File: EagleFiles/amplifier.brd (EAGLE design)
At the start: 100 x 80 mm, 52 parts, among them X1 736880-49

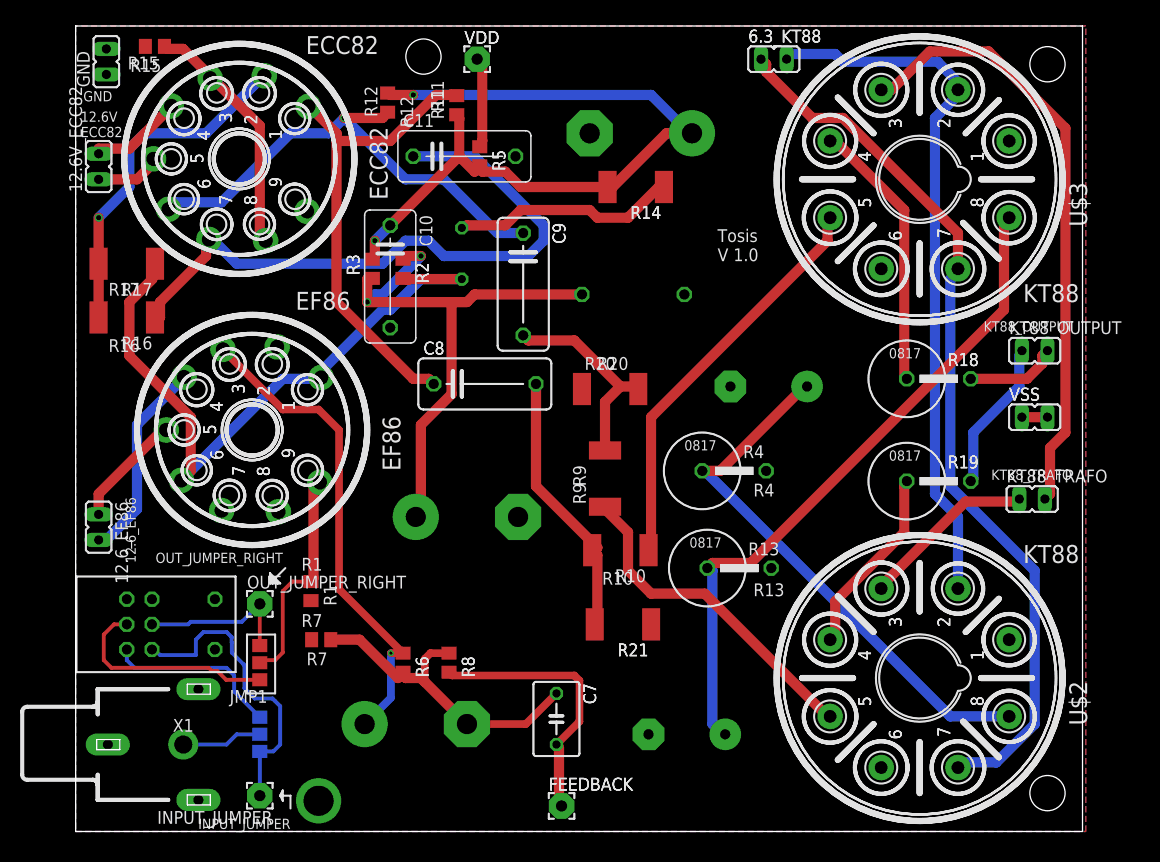
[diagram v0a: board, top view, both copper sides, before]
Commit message: last not good design.
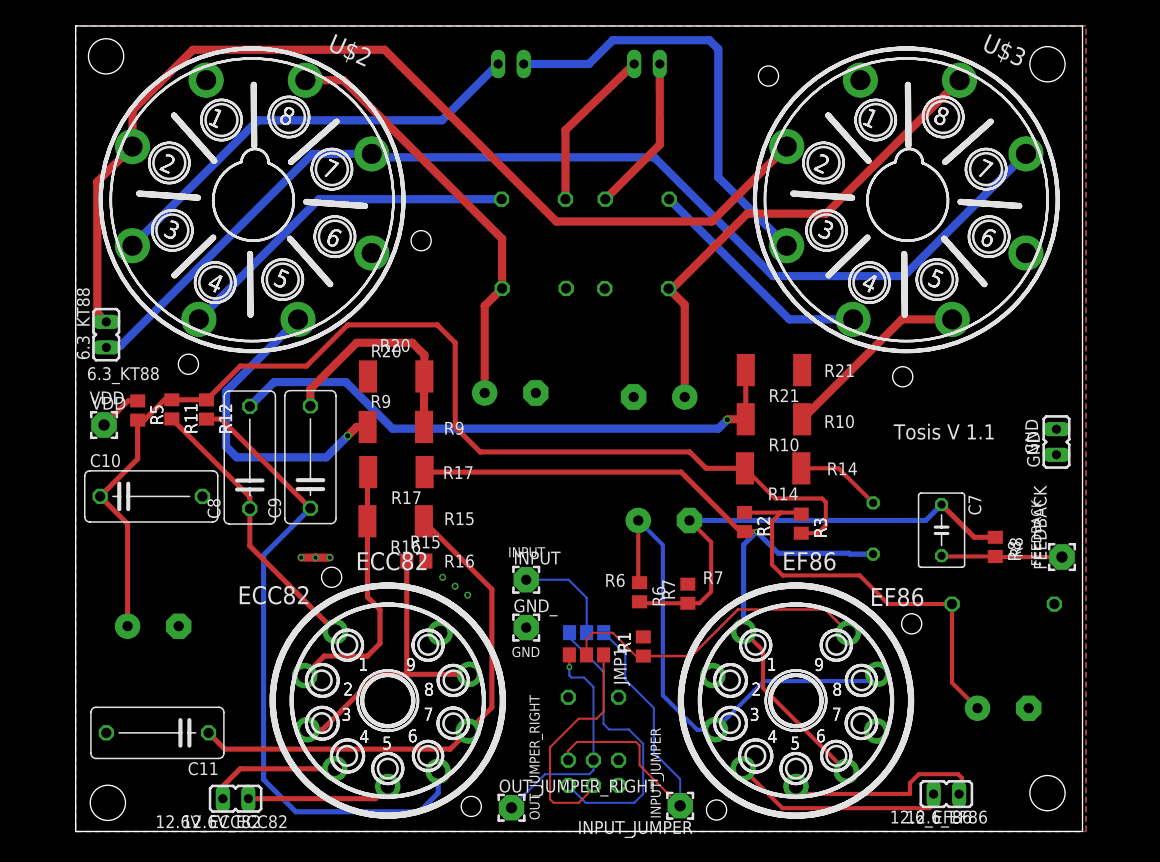
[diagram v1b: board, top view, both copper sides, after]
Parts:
- removed VSS: (no value), jumper:JP1
- removed X1: 736880-49, con-conrad:736880-49
- added GND_, INPUT: (no value), wirepad:2,54/1,0
- C1: device resistor:EB20D -> rcl:E5-13
- C12: value 100mF/100V -> 100u/100V; device rcl:E7,5-18 -> rcl:E5-10,5
- C2: value 10m/25V -> 10u/25V; device resistor:EB20D -> rcl:E5-8,5
- C3: value 10m -> 10u/450V; device resistor:EB20D -> rcl:E5-13
- C4: value 100uF/100V -> 100u/100V; device rcl:E7,5-18 -> rcl:E5-10,5
- C5: value 100nF -> 100n
- U$2, U$3: value KT88 -> KT88OKTAL1; device Tubes_all:OKTAL -> tubes_stockes:OKTAL1
- moved GND 101.6 mm to (97.4, 38.7)
- moved 12.6_EF86 88.3 mm to (86.5, 3.71), turned to 90 degrees
- moved U$2 81.6 mm to (17.5, 62.7), turned to 156 degrees
- moved 6.3_KT88 71.7 mm to (3.04, 49.3), turned to 0 degrees
- moved C3 68.9 mm to (7.70, 20.4), turned to 180 degrees
- moved KT88_TRAFO 67.4 mm to (43.2, 76.2), flipped to the bottom, turned to 90 degrees
- moved C11 64.9 mm to (8.12, 9.79), turned to 180 degrees
- moved 12.6V_ECC82 64.2 mm to (15.9, 3.26), turned to 90 degrees
- moved EF86 60.3 mm to (71.5, 13.0), turned to 180 degrees
- moved R15 57.3 mm to (33.8, 26.9), turned to 0 degrees
- moved C1 56.5 mm to (92.1, 12.2)
- moved ECC82 55.8 mm to (31.0, 13.0), turned to 180 degrees
- moved FEEDBACK 55.5 mm to (98.0, 27.3), turned to 90 degrees
- moved R8 55.5 mm to (91.3, 28.3)
- moved VDD 51.9 mm to (2.82, 40.4)
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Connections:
- removed net N$30: VSS.1, VSS.2
- removed net N$35: C2.+, EF86.3, R6.1
- net GND: now also GND_.1; no longer X1.1, X1.1@1, X1.1@2
- net N$1: now also INPUT.1; no longer X1.2
- net N$36: now also C2.+, EF86.3, R6.1
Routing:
- net N$36: track 0.00 -> 49.7 mm
- net N$35: track 49.0 -> 0.00 mm, vias 1 -> 0
- net N$7: track 77.6 -> 112.7 mm, vias 2 -> 0
- net N$15: track 27.2 -> 57.4 mm, vias 0 -> 1
- net N$34: track 70.6 -> 100.5 mm
- net KT88: track 17.7 -> 43.8 mm
- net N$17: track 40.6 -> 19.0 mm
- net N$33: track 89.4 -> 109.4 mm
- net N$14: track 47.5 -> 27.8 mm
- net N$18: track 67.2 -> 48.9 mm
- net KT88_2: track 60.7 -> 43.0 mm
- net N$10: track 48.5 -> 64.4 mm, vias 1 -> 0
- net N$23: track 19.2 -> 35.0 mm
- net N$3: track 32.7 -> 48.0 mm
- net N$6: track 56.7 -> 42.1 mm, vias 2 -> 0
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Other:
- board text added: "12.6V_ECC82"
- board text added: "INPUT"
- board text added: "Tosis V 1.1"
- board text removed: "12.6V ECC82"
- board text removed: "KT88"
- board text removed: "Tosis V 1.0"
- board text removed: "VSS"
